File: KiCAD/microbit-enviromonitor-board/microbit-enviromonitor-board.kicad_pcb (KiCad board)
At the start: 2 copper layers, 45.7 x 62.2 mm, 12 parts, among them J1 12V, J2 SERIAL, J3 3V3, J4 PUMP, Q1 TIP41C, U1 REGULATOR

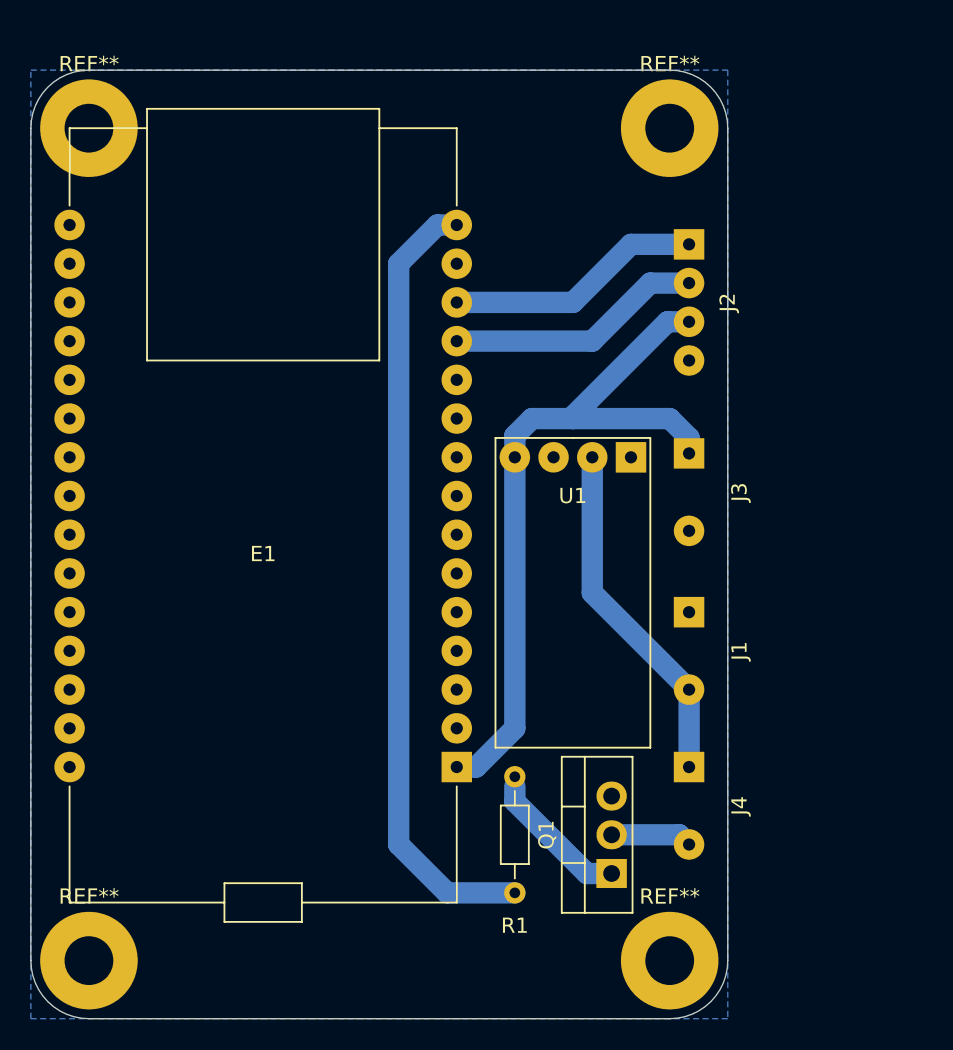
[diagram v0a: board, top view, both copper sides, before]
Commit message: Board changes
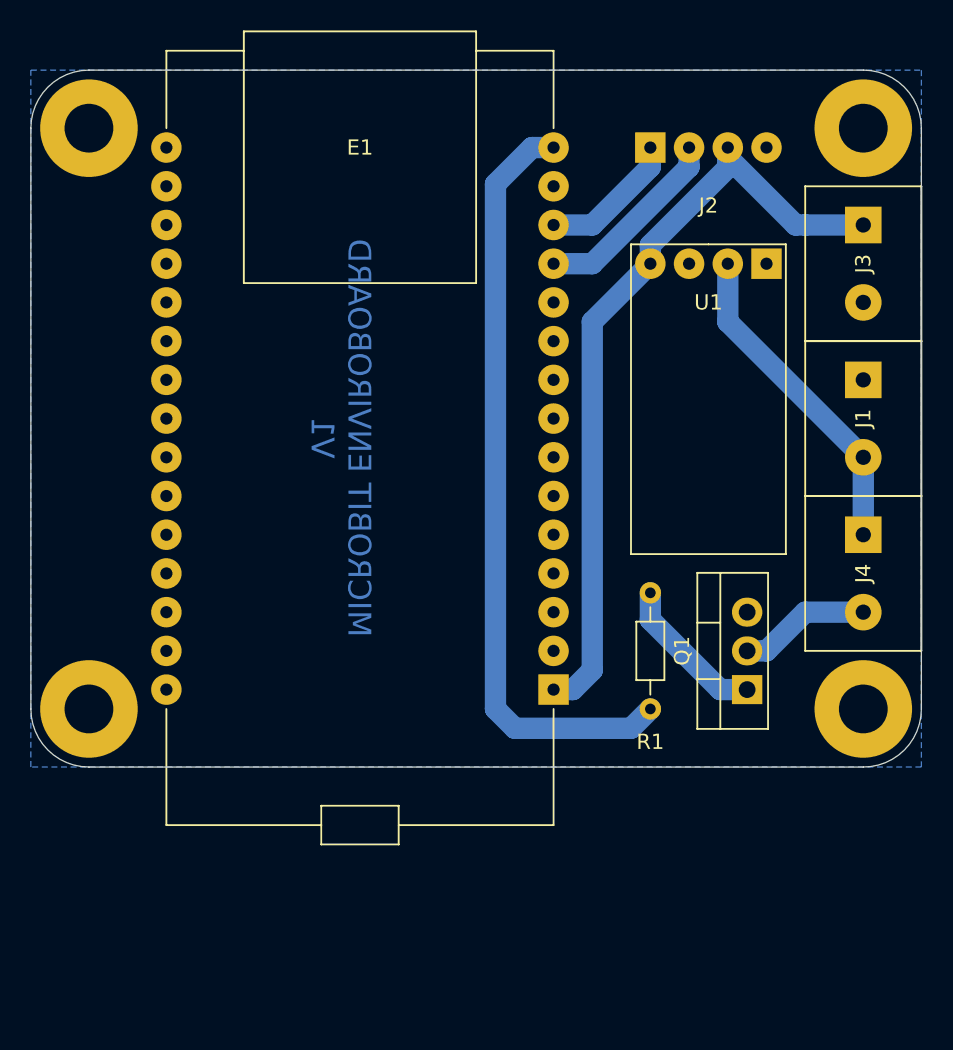
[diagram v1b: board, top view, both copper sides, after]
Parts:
- removed the REF** at (3.81, 58.4)
- removed the REF** at (41.9, 58.4)
- removed the REF** at (41.9, 3.81)
- added REF**: MountingHole_3.2mm_M3_Pad, MountingHole:MountingHole_3.2mm_M3_Pad, F.Cu at (3.81, 41.9)
- added REF**: MountingHole_3.2mm_M3_Pad, MountingHole:MountingHole_3.2mm_M3_Pad, F.Cu at (54.6, 41.9)
- added REF**: MountingHole_3.2mm_M3_Pad, MountingHole:MountingHole_3.2mm_M3_Pad, F.Cu at (54.6, 3.81)
- J1, J3, J4: footprint headers:2_double_spaced -> headers:screw_terminal
- moved J1 19.1 mm to (54.6, 22.9)
- moved J4 19.0 mm to (54.6, 33.0)
- moved J3 18.8 mm to (54.6, 12.7)
- moved U1 15.5 mm to (44.5, 12.7)
- moved Q1 15.0 mm to (47.0, 40.6)
- moved R1 15.0 mm to (40.6, 34.3)
- moved J2 10.2 mm to (44.5, 5.08), turned to 0 degrees
- moved E1 8.13 mm to (21.6, 24.1)
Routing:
- net Net-(E1-Pad13): track 16.8 -> 9.34 mm
- net +3V3: track 47.8 -> 52.4 mm
- net Net-(E1-Pad12): track 16.8 -> 12.6 mm
- net Net-(J4-Pad2): track 5.34 -> 8.67 mm
- net +12V: track 23.0 -> 21.5 mm
- net /PUMP: track 51.9 -> 50.4 mm
- net Net-(Q1-Pad1): track 9.30 -> 10.0 mm
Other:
- board size 45.7 x 62.2 mm -> 58.4 x 45.7 mm
- board text added: "MICROBIT ENVIROBOARD V1"
